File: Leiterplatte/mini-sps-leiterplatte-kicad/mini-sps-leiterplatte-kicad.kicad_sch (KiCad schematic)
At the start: 17 parts, among them J1 Conn_01x03_Socket, J2 Conn_01x03_Socket, J3 Conn_01x03_Socket, K1 SRD-05VDC-SL-C, K2 SRD-05VDC-SL-C, K3 SRD-05VDC-SL-C

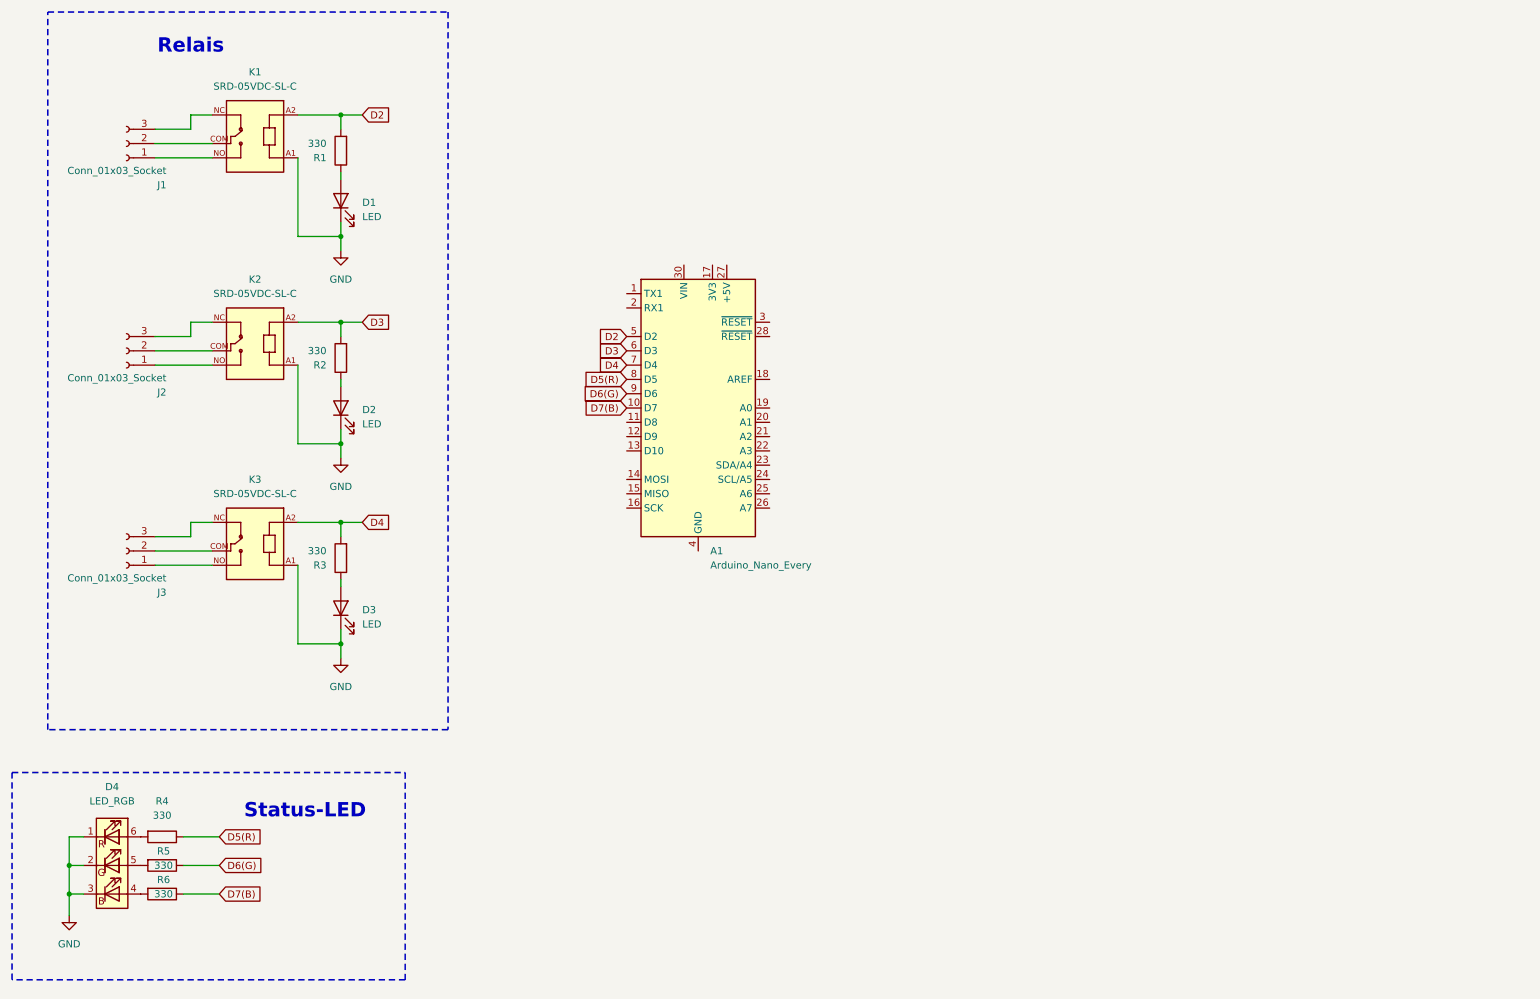
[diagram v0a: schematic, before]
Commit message: v.2 schreubdinger
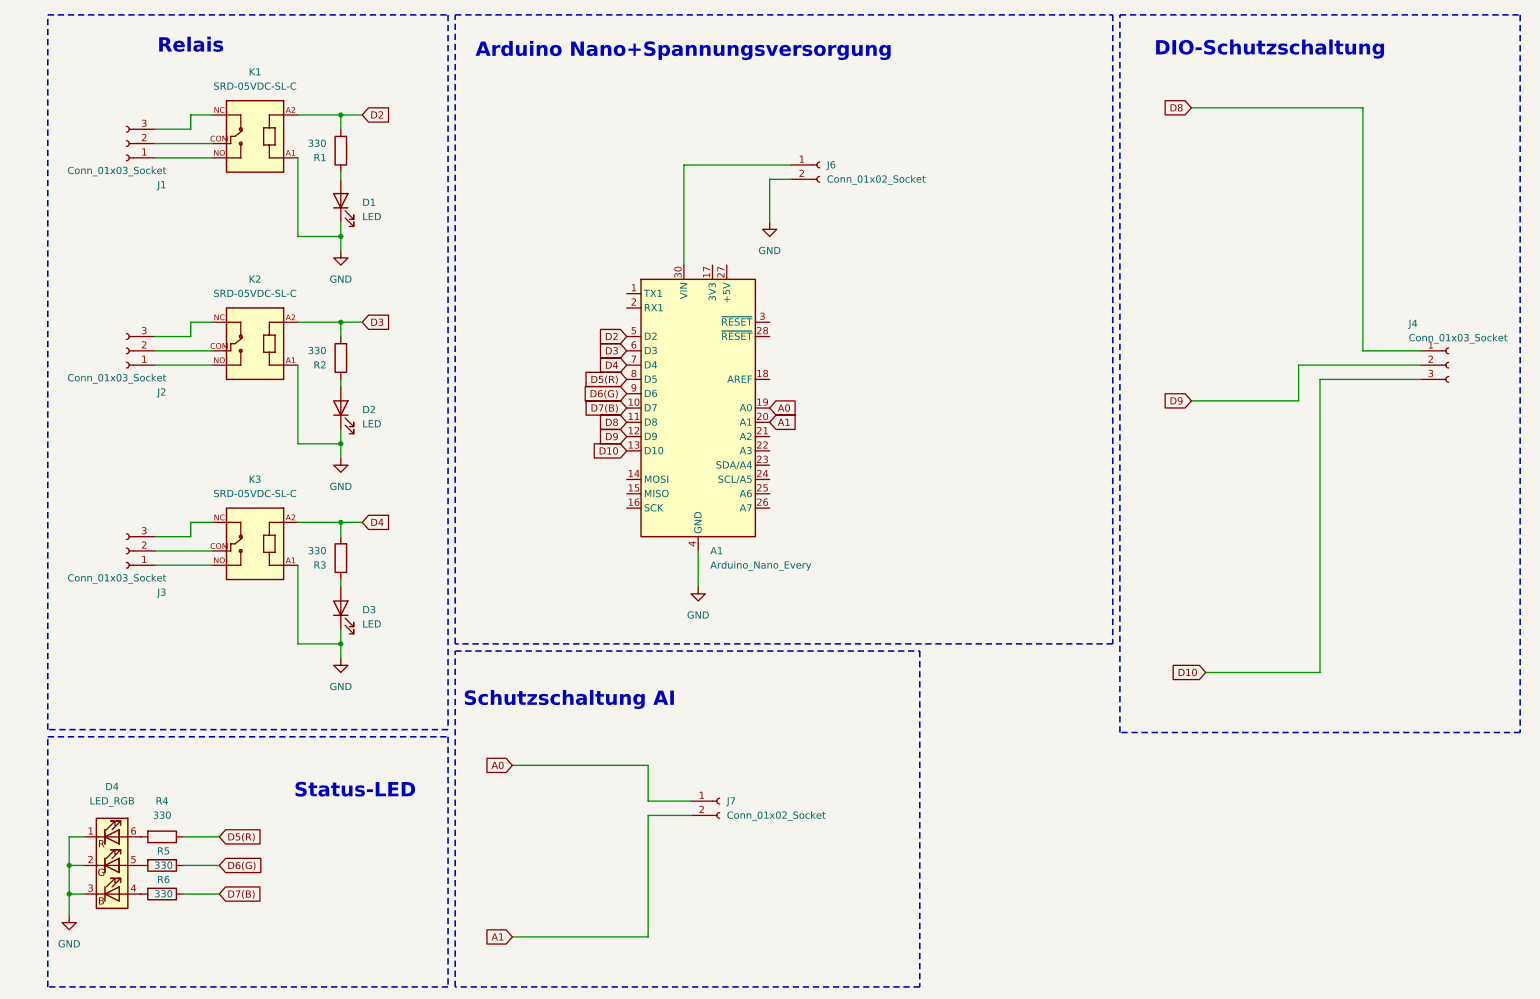
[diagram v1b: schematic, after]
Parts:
- added J4: Conn_01x03_Socket, TerminalBlock:TerminalBlock_Altech_AK300-3_P5.00mm, symbol Connector:Conn_01x03_Socket
- added J6, J7: Conn_01x02_Socket, TerminalBlock:TerminalBlock_Altech_AK300-2_P5.00mm, symbol Connector:Conn_01x02_Socket
- D1, D2, D3: footprint (none) -> LED_THT:LED_D5.0mm
- D4: footprint (none) -> LED_THT:LED_D5.0mm-4_RGB_Wide_Pins
- J1, J2, J3: footprint (none) -> TerminalBlock:TerminalBlock_Altech_AK300-3_P5.00mm
- K1, K2, K3: footprint SRD-05VDC-SL-C:RELAY_SRD-05VDC-SL-C -> custom:RELAY_SRD-05VDC-SL-C
- R1, R2, R3, R4, R5, R6: footprint (none) -> Resistor_THT:R_Axial_DIN0207_L6.3mm_D2.5mm_P10.16mm_Horizontal
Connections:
- net GND: now also A1.29 (GND), A1.4 (GND), J6.2 (Pin_2)
- net D8: now reaches A1.11 (D8)
- net D8: now also J4.1 (Pin_1)
- net D9: now reaches A1.12 (D9)
- net D9: now also J4.2 (Pin_2)
- net D10: now reaches A1.13 (D10)
- net D10: now also J4.3 (Pin_3)
- net A0: now reaches A1.19 (A0)
- net A0: now also J7.1 (Pin_1)
- net A1: now reaches A1.20 (A1)
- net A1: now also J7.2 (Pin_2)
- net at A1.30 (VIN): now also J6.1 (Pin_1)
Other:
- note added: "Arduino Nano+Spannungsversorgung"
- note added: "DIO-Schutzschaltung"
- note added: "Schutzschaltung AI"
